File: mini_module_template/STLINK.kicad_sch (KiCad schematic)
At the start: 25 parts, among them U6 STM32F103CB, Y2 8MHz

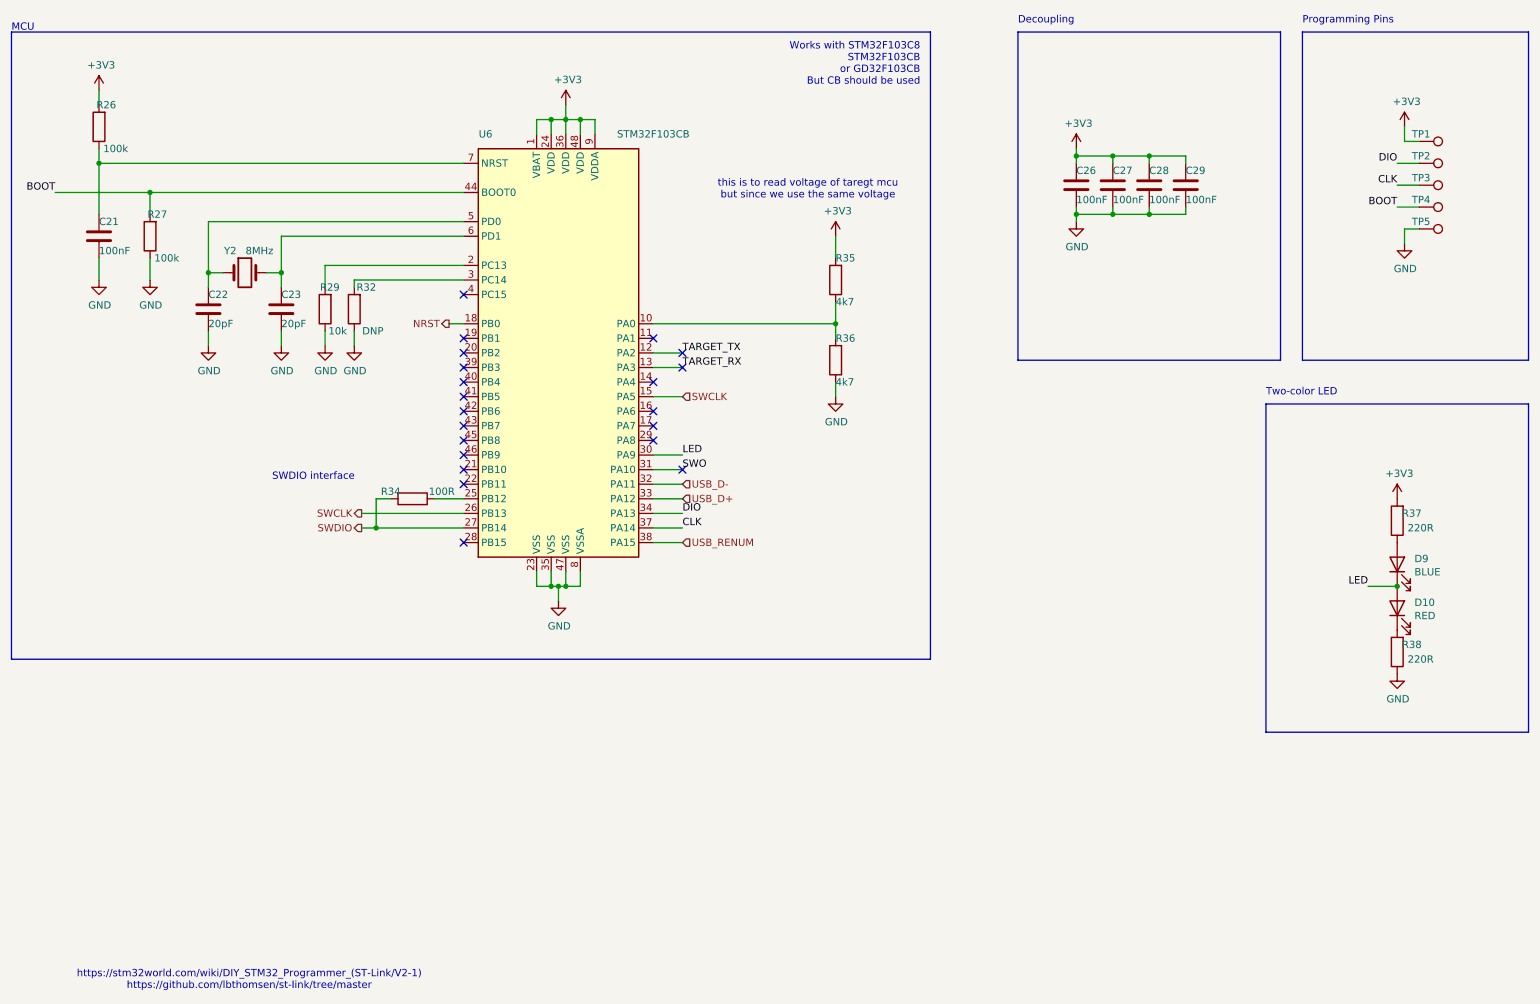
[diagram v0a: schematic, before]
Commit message: Leyout rev 1
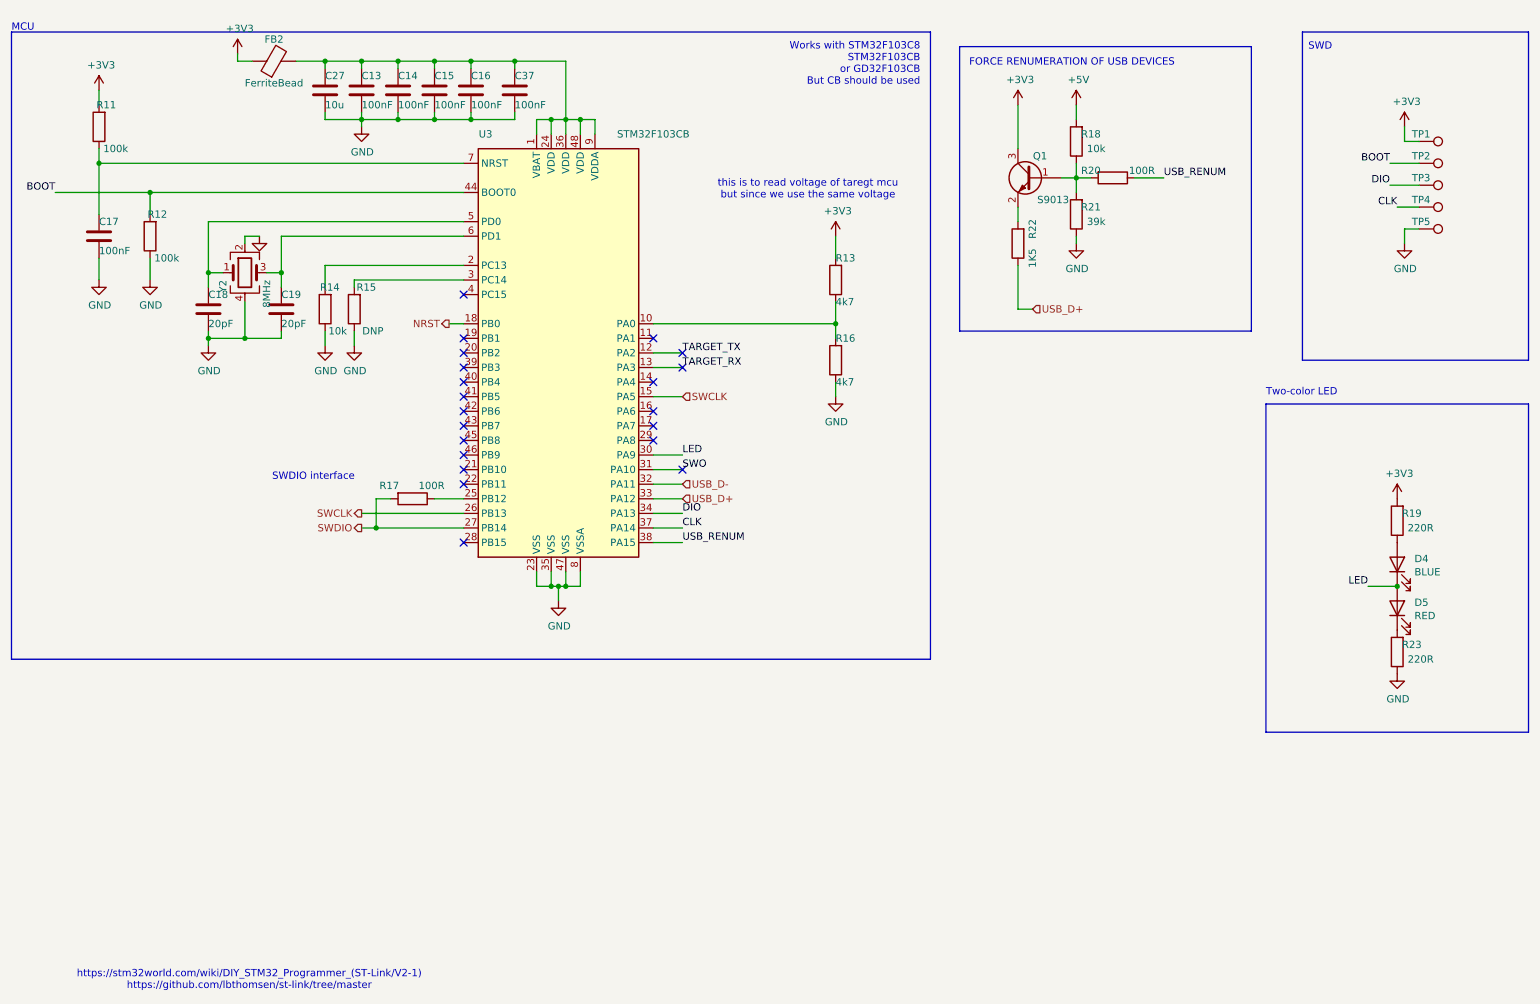
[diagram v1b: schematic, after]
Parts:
- removed Y2: 8MHz, st-link:Crystal_SMD_5032-2Pin_5.0x3.2mm, symbol Device:Crystal
- added C27: 10u, Capacitor_SMD:C_0805_2012Metric, symbol Device:C
- added C37: 100nF, Capacitor_SMD:C_0402_1005Metric, symbol Device:C
- added FB2: FerriteBead, Inductor_SMD:L_0805_2012Metric, symbol Device:FerriteBead
- added Q1: S9013, Package_TO_SOT_SMD:SOT-23, symbol Device:Q_NPN_BEC
- added R18: 10k, Resistor_SMD:R_0402_1005Metric, symbol Device:R
- added R20: 100R, Resistor_SMD:R_0402_1005Metric, symbol Device:R
- added R21: 39k, Resistor_SMD:R_0402_1005Metric, symbol Device:R
- added R22: 1K5, Resistor_SMD:R_0402_1005Metric, symbol Device:R
- added Y2: 8MHz, Crystal:Crystal_SMD_3225-4Pin_3.2x2.5mm, symbol Device:Crystal_GND24
- R17: renamed from R34; footprint Resistor_SMD:R_0402_1005Metric -> Resistor_SMD:R_0603_1608Metric
- renumbered C26 to C13, C27 to C14, C28 to C15, C29 to C16, C21 to C17, C22 to C18, C23 to C19, D9 to D4, D10 to D5, R26 to R11, R27 to R12, R35 to R13, R29 to R14, R32 to R15, R36 to R16, R37 to R19, R38 to R23, U6 to U3
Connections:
- net +3V3: now also FB2.1, Q1.3 (C); no longer C13.1, C14.1, C15.1, C16.1, U3.1 (VBAT), U3.24 (VDD), U3.36 (VDD), U3.48 (VDD), U3.9 (VDDA)
- net BOOT: now also TP2.1; no longer TP4.1
- net CLK: now also TP4.1; no longer TP3.1
- net DIO: now also TP3.1; no longer TP2.1
- net GND: now also C27.2, C37.2, R21.1, Y2.2, Y2.4
- net USB_D+: now also R22.1
- net USB_RENUM: now also R20.1
- net at C19.1, U3.6 (PD1): now also Y2.3
- net at C18.1, U3.5 (PD0): now also Y2.1
- new net: C13.1, C14.1, C15.1, C16.1, C27.1, C37.1, FB2.2, U3.1 (VBAT), U3.24 (VDD), U3.36 (VDD), U3.48 (VDD), U3.9 (VDDA)
- new net: Q1.2 (E), R22.2
- new net: Q1.1 (B), R18.1, R20.2, R21.2
- new net +5V: R18.2
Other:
- note added: "FORCE RENUMERATION OF USB DEVICES"
- note added: "SWD"
- note removed: "Decoupling"
- note removed: "Programming Pins"
- moved on the sheet: C13, C14, C15, C16
